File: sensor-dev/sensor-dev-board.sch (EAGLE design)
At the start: 50 parts, among them IC1 REG1117, P1 B4B-PH-K, P2 B4B-PH-K, U1 ATMEGA328PB-AUR

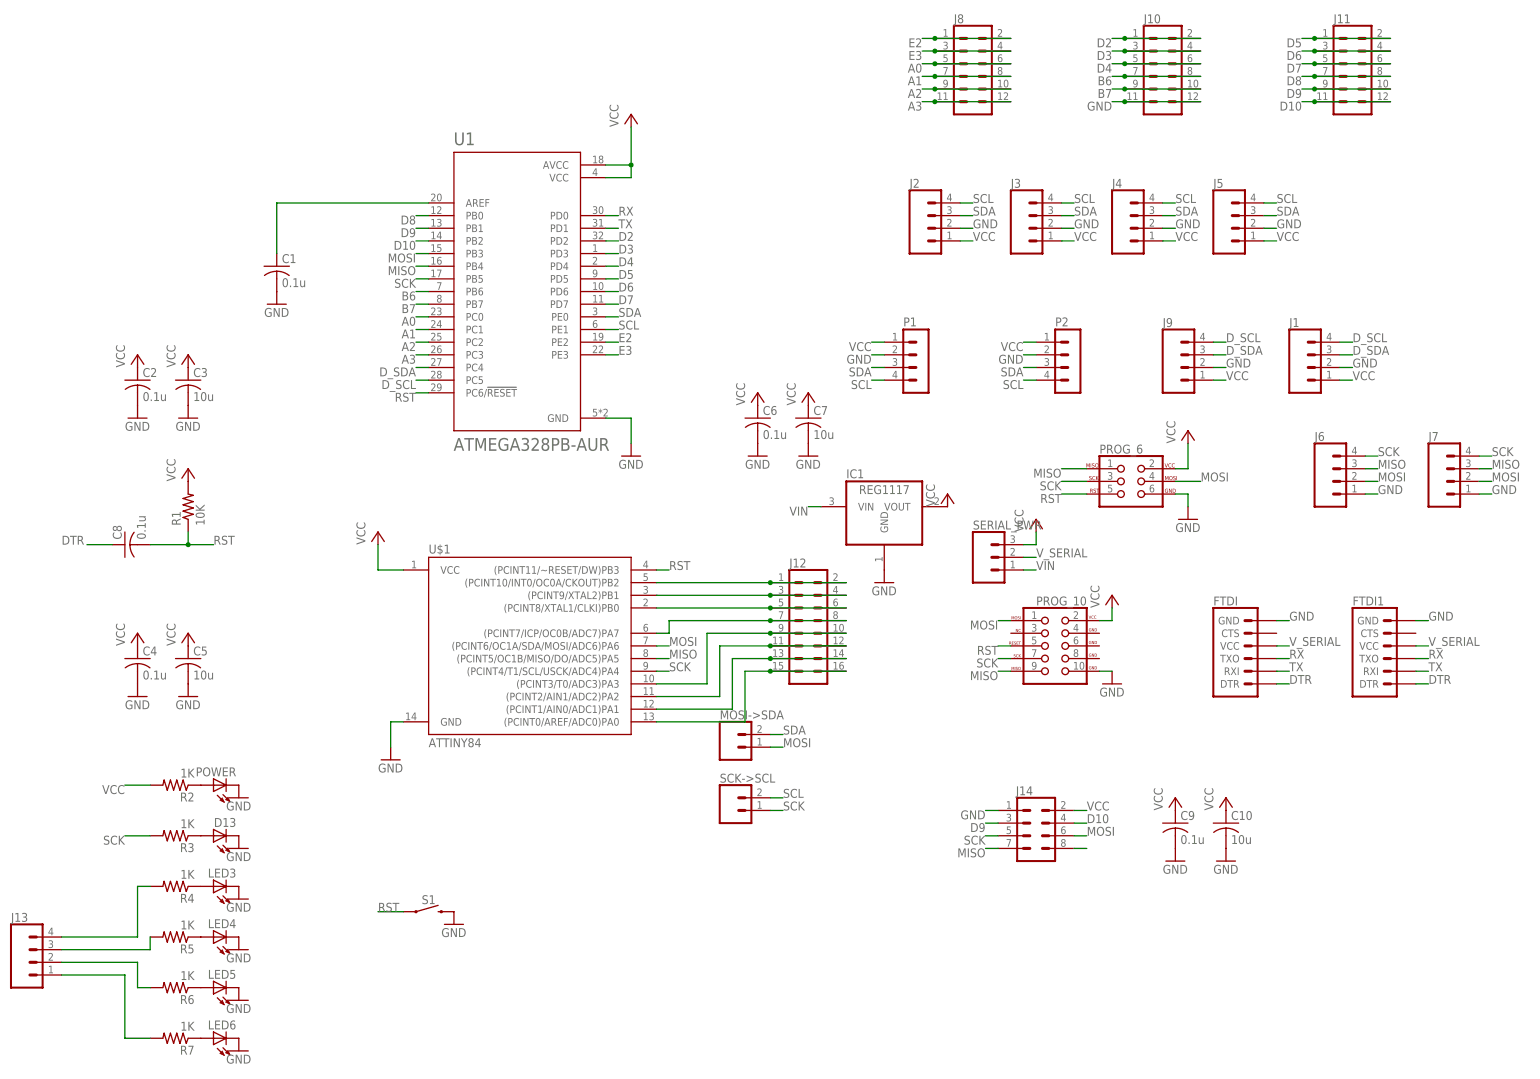
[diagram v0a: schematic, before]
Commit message: Sensor dev board 1.4
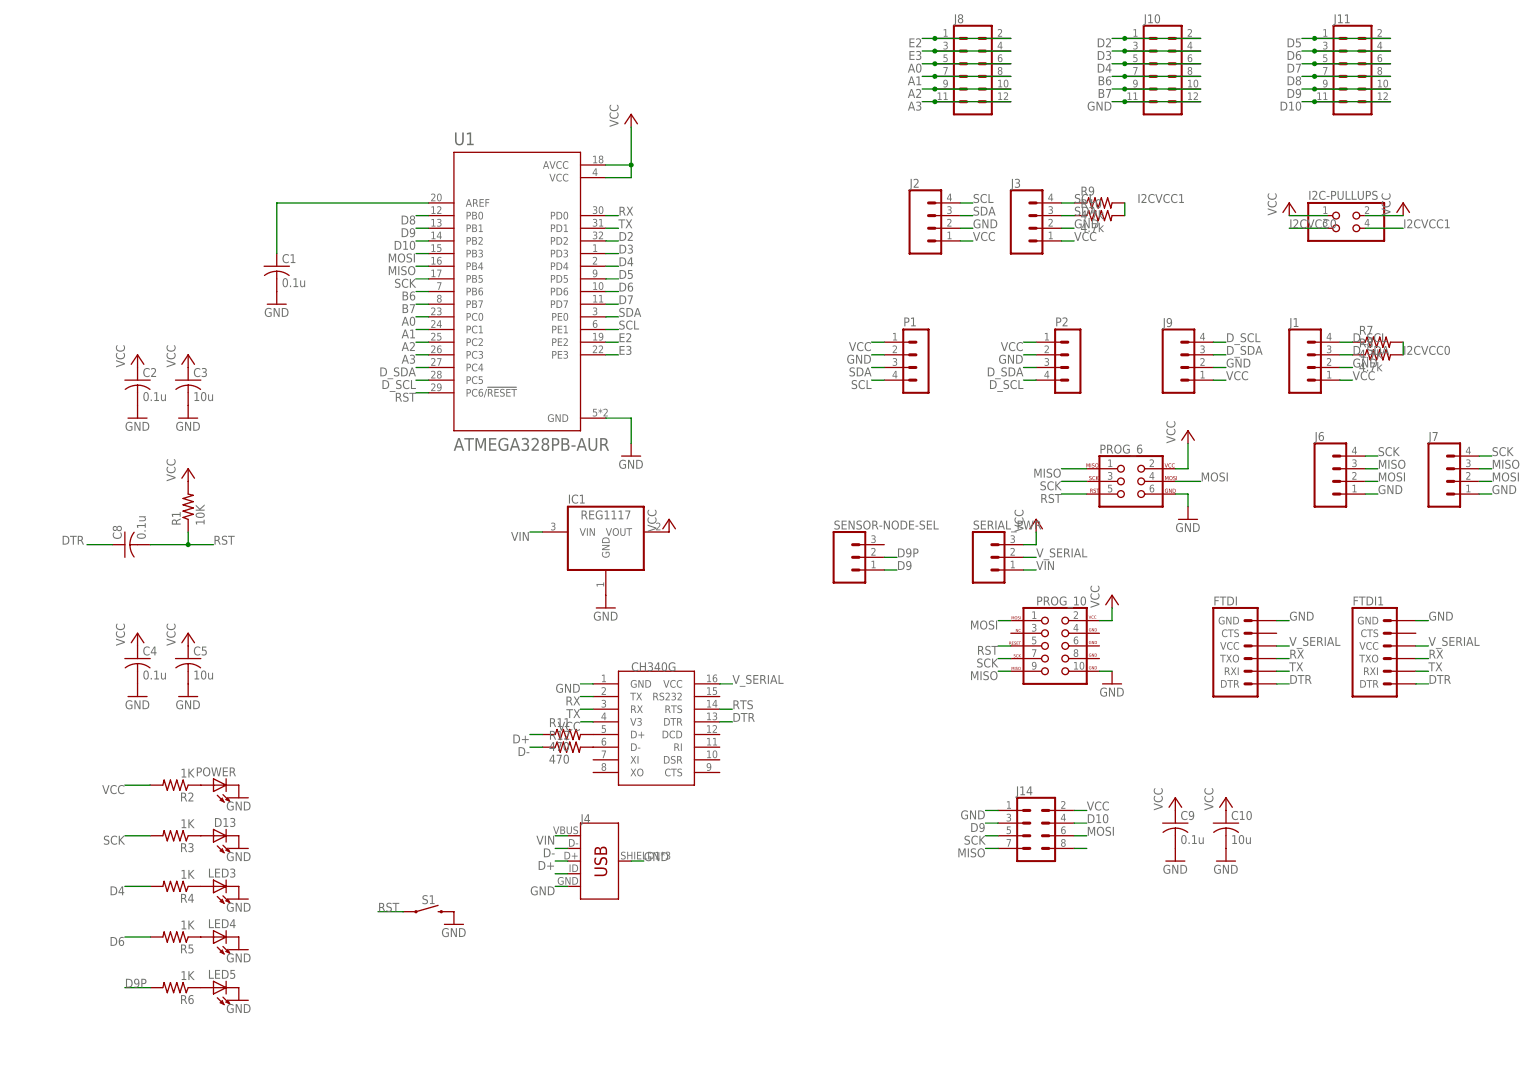
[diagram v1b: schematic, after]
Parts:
- removed C6: 0.1u, rcl:C-USC1206
- removed C7: 10u, rcl:C-USC1206
- removed J12: (no value), SparkFun-Connectors:CONN_08X2
- removed J13, J5: (no value), SparkFun-Connectors:CONN_04
- removed LED6: (no value), led:LEDSML1206
- removed MOSI->SDA, SCK->SCL: (no value), SparkFun-Connectors:CONN_02
- removed U$1: ATTINY84, SparkFun-IC-Microcontroller:ATTINY84
- added CH340C: CH340C, ch340g:CH340G
- added I2C-PULLUPS: (no value), pinhead:PINHD-2X2
- added R10, R8, R9: 4.7k, resistor:R-US_R1206
- added R11, R12: 470, resistor:R-US_R1206
- added SENSOR-NODE-SEL: (no value), SparkFun-Connectors:CONN_03
- J4: device SparkFun-Connectors:CONN_04 -> SparkFun-Connectors:USB_MICRO-B_FEMALE-SMT
- R7: value 1K -> 4.7k
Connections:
- removed net N$15: LED6.A, R7.1
- removed net N$18: J13.3, R5.2
- removed net N$19: J13.4, R4.2
- removed net N$20: J13.2, R6.2
- removed net N$21: J13.1, R7.2
- removed net N$3: J12.3, J12.4, U$1.(PCINT9/XTAL2)PB1
- removed net N$4: J12.5, J12.6, U$1.(PCINT8/XTAL1/CLKI)PB0
- removed net N$6: J12.10, J12.9, U$1.(PCINT3/T0/ADC3)PA3
- removed net N$7: J12.11, J12.12, U$1.(PCINT2/AIN1/ADC2)PA2
- removed net N$8: J12.13, J12.14, U$1.(PCINT1/AIN0/ADC1)PA1
- new net D+: J4.D+, R11.1
- new net D-: J4.D-, R12.1
- new net D9P: R6.2, SENSOR-NODE-SEL.2
- new net I2CVCC0: I2C-PULLUPS.3, R7.2, R8.2
- new net I2CVCC1: I2C-PULLUPS.4, R10.2, R9.2
- new net RTS: CH340C.RTS
- net D4: now also R4.2
- net D6: now also R5.2
- net D9: now also SENSOR-NODE-SEL.1
- net DTR: now also CH340C.DTR
- net D_SCL: now also P2.4, R7.1
- net D_SDA: now also P2.3, R8.1
- net GND: now also CH340C.GND, J4.GND, J4.SHIELD; no longer C6.2, C7.2, J4.2, J5.2, LED6.C, U$1.GND
- net MISO: no longer U$1.(PCINT5/OC1B/MISO/DO/ADC5)PA5
- net MOSI: no longer MOSI->SDA.1, U$1.(PCINT6/OC1A/SDA/MOSI/ADC6)PA6
- net N$1: now also CH340C.D+, R11.2; no longer J12.1, J12.2, U$1.(PCINT10/INT0/OC0A/CKOUT)PB2
- net N$2: now also CH340C.D-, R12.2; no longer J12.7, J12.8, U$1.(PCINT7/ICP/OC0B/ADC7)PA7
- net N$9: now also J4.ID; no longer J12.15, J12.16, U$1.(PCINT0/AREF/ADC0)PA0
- net RST: no longer U$1.(PCINT11/~RESET/DW)PB3
- net RX: now also CH340C.TX
- net SCK: no longer SCK->SCL.1, U$1.(PCINT4/T1/SCL/USCK/ADC4)PA4
- net SCL: now also R9.1; no longer J4.4, J5.4, P2.4, SCK->SCL.2
- net SDA: now also R10.1; no longer J4.3, J5.3, MOSI->SDA.2, P2.3
- net TX: now also CH340C.RX
- net VCC: now also CH340C.V3, I2C-PULLUPS.1, I2C-PULLUPS.2; no longer C6.1, C7.1, J4.1, J5.1, U$1.VCC
- net VIN: now also J4.VBUS
- net V_SERIAL: now also CH340C.VCC
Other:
- moved on the sheet: IC1, R7
